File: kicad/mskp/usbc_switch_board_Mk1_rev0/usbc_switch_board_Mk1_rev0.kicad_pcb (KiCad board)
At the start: 2 copper layers, 27 parts, among them J1 USB_C_Receptacle_USB2.0_14P, J2 USB_C_Receptacle_USB2.0_14P, J3 USB_A, J4 USB_out_pads, J5 switch_ctrl_pads, Q1 2N3906, Q2 2N3904, U1 FSUSB42MUX, U2 AMS1117-3.3

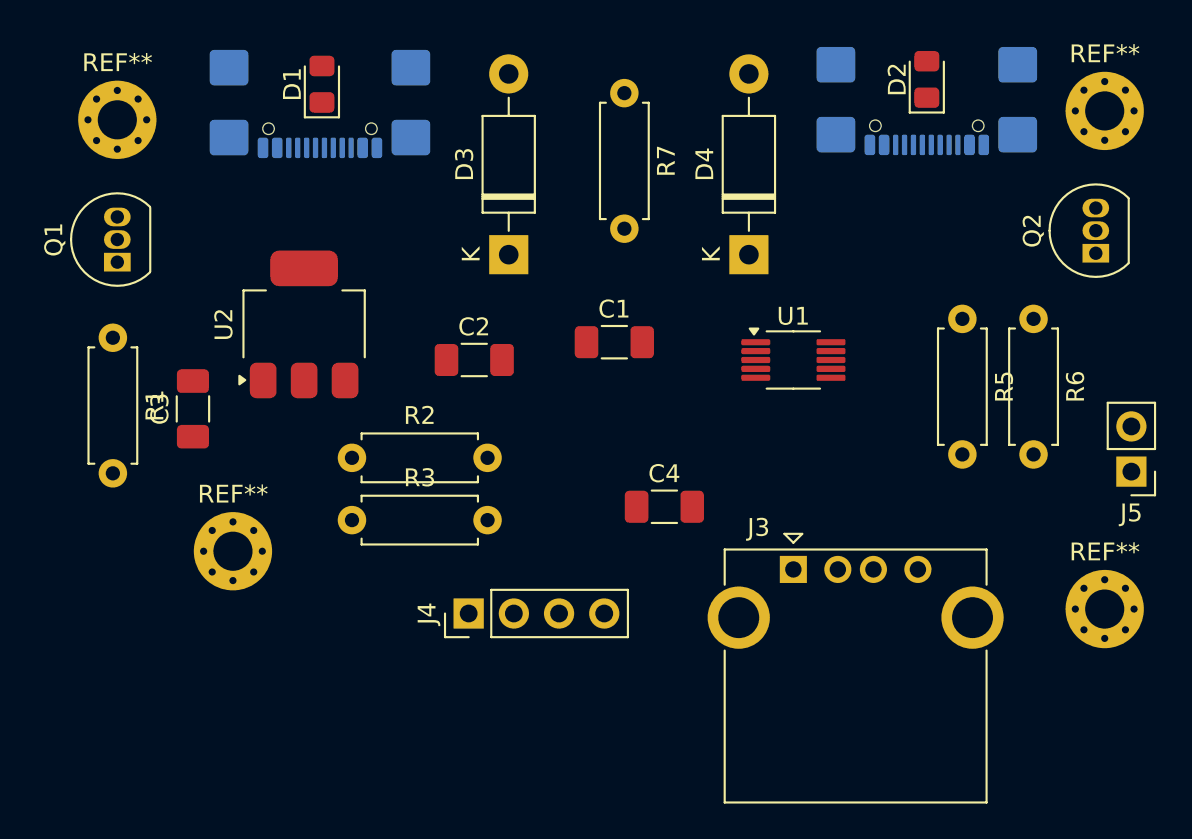
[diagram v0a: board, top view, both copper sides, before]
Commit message: Continues work with rough PCB outlines
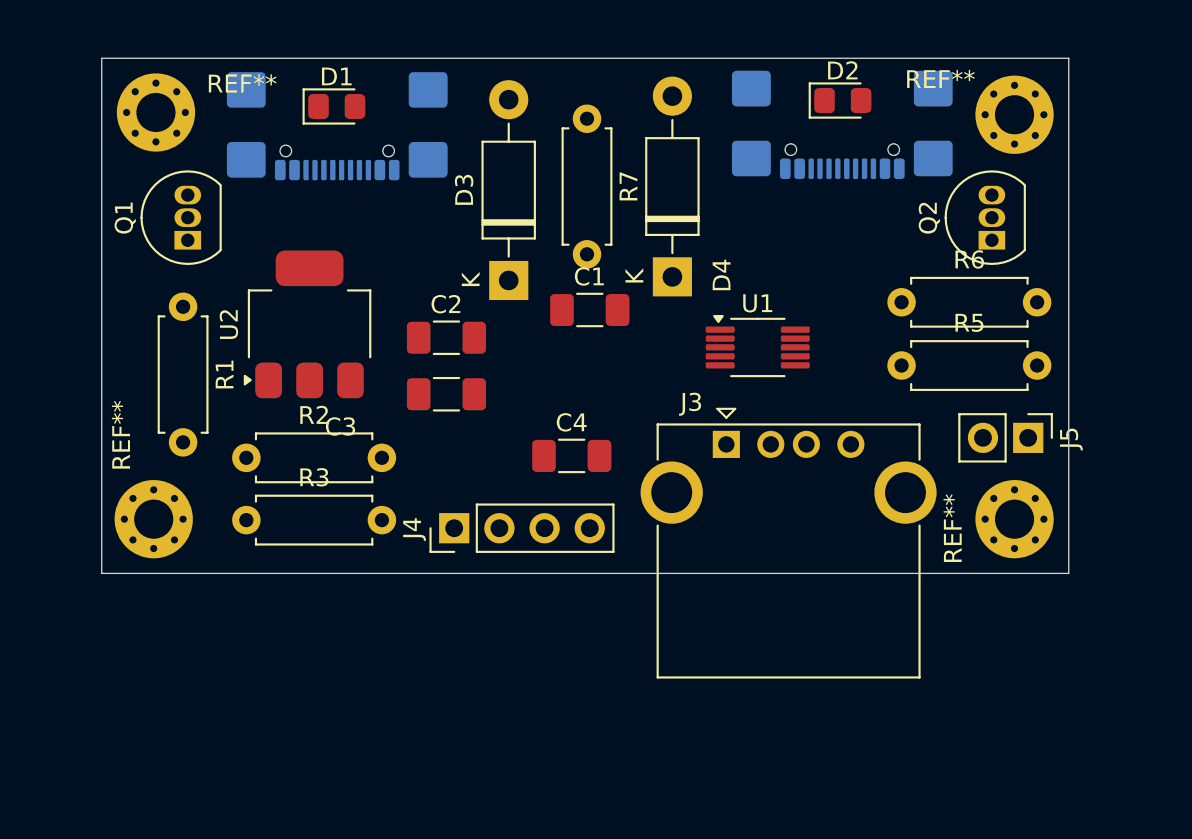
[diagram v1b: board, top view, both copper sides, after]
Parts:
- moved C3 14.3 mm to (122.5, 84.9), turned to 180 degrees
- moved J3 7.97 mm to (138.2, 87.7)
- moved R6 7.48 mm to (148.1, 79.8), turned to 0 degrees
- moved REF** 7.16 mm to (154.4, 91.9)
- moved J5 6.10 mm to (155.2, 87.4), turned to -90 degrees
- moved C4 5.94 mm to (129.5, 88.4)
- moved R2 5.94 mm to (111.3, 88.5)
- moved R3 5.94 mm to (111.3, 92.0)
- moved Q2 5.89 mm to (153.2, 76.3)
- moved REF** 5.07 mm to (154.4, 69.2)
- moved J2 4.94 mm to (144.8, 68.6)
- moved D2 4.87 mm to (144.8, 68.4), turned to 0 degrees
- moved J4 4.86 mm to (122.9, 92.5)
- moved REF** 4.80 mm to (106.0, 91.9)
- moved D4 4.48 mm to (135.2, 78.3)
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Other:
- board outline added: 54.4 x 29 mm
